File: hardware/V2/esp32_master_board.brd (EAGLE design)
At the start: 65 x 35 mm, 62 parts, among them IC1 SN74HC138PW, IC2 MAX17502EATB+T, SW1 B3U-1000P-2P-SMD

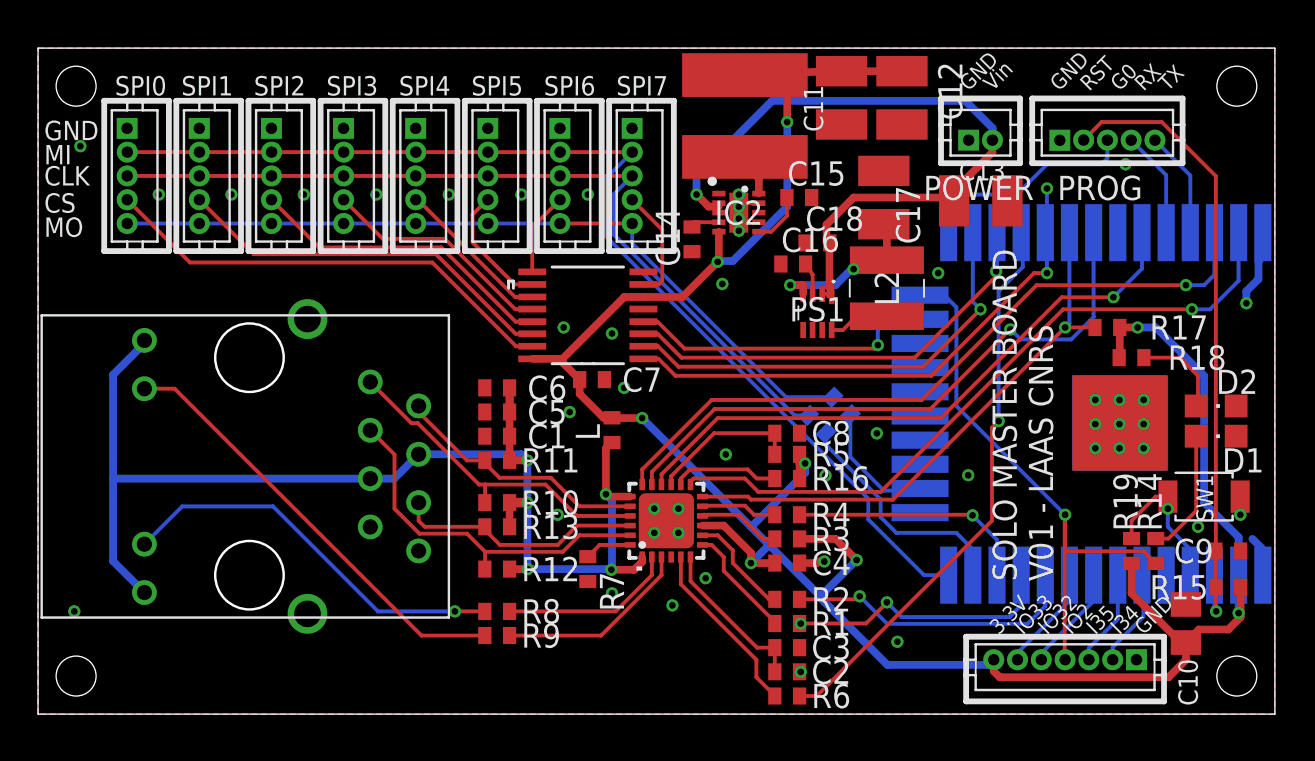
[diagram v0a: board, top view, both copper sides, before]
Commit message: [HARDWARE] Continue V2 design
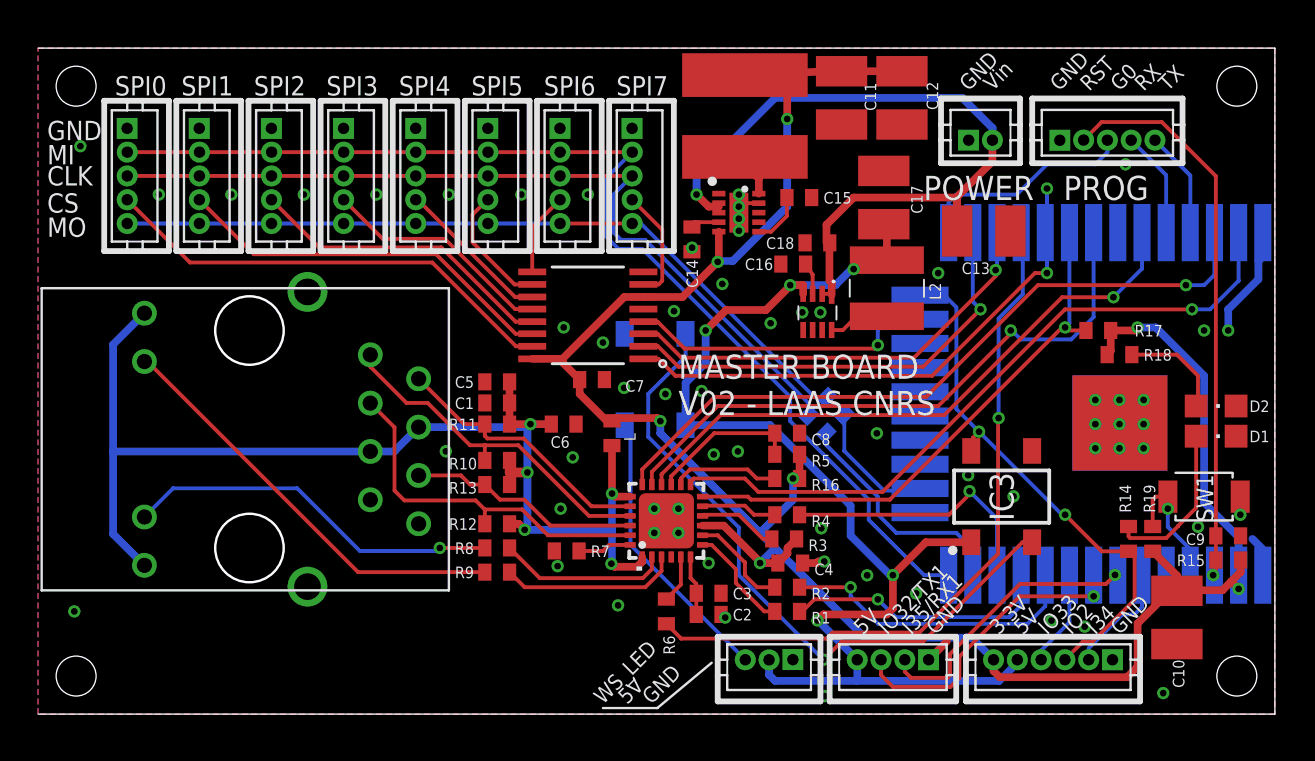
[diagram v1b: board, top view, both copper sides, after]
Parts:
- added IC3, IC4: WS2812B, WS2812B:WS2812B
- added U$5: DF13-3P-1.25DSA, con-hirose-df13:DF13-3P-1.25DSA
- added U$6: DF13-4P-1.25DSA, con-hirose-df13:DF13-4P-1.25DSA
- C10: device resistor:C0805K -> resistor:C1210
- C17: value 1u -> 22u
- U$4: value DF13-7P-1.25DSA -> DF13-6P-1.25DSA; device con-hirose-df13:DF13-7P-1.25DSA -> con-hirose-df13:DF13-6P-1.25DSA
- moved R6 7.75 mm to (33.0, 5.40), turned to 90 degrees
- moved C2 5.11 mm to (35.2, 5.24)
- moved C3 5.02 mm to (35.2, 6.35)
- moved C6 3.98 mm to (27.6, 15.2), turned to 0 degrees
- moved R8 3.33 mm to (24.1, 8.73)
- moved R9 3.33 mm to (24.1, 7.46)
- moved R12 2.38 mm to (24.1, 10.0)
- moved R10 2.22 mm to (24.1, 13.3)
- moved R13 2.22 mm to (24.1, 12.1)
- moved R11 1.90 mm to (24.1, 15.2)
- moved C1 1.75 mm to (24.1, 16.4)
- moved C13 1.60 mm to (49.7, 25.4)
- moved C5 1.59 mm to (24.1, 17.5)
- moved R14 1.56 mm to (57.3, 9.21)
- moved R7 1.46 mm to (27.8, 8.57), turned to 0 degrees
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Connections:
- removed net I35: U$1.IO35, U$4.P$3
- removed net IO32: U$1.IO32, U$4.P$5
- new net I35_RX1: U$1.IO35, U$6.P$2
- new net IO32_TX1: U$1.IO32, U$6.P$3
- new net N$19: IC3.2, IC4.4
- new net WSLED_OUT: IC4.2, U$5.P$3
- net 5V: now also IC3.1, IC4.1, U$4.P$5, U$5.P$2, U$6.P$4
- net GND: now also IC3.3, IC4.3, U$5.P$1, U$6.P$1
- net IO2: now also IC3.4, U$4.P$3; no longer U$4.P$4
- net IO33: now also U$4.P$4; no longer U$4.P$6
- net VCC: now also U$4.P$6; no longer U$4.P$7
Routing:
- net 5V: track 8.72 -> 64.1 mm, vias 2 -> 5
- net N$19: track 0.00 -> 35.3 mm, vias 0 -> 1
- net IO32_TX1: track 0.00 -> 16.0 mm, vias 0 -> 1
- net WSLED_OUT: track 0.00 -> 15.0 mm
- net I35_RX1: track 0.00 -> 14.9 mm, vias 0 -> 1
- net VCC: track 127.1 -> 118.9 mm, vias 8 -> 7
- net CLK50: track 29.8 -> 37.1 mm
- net N$5: track 9.35 -> 2.52 mm
- net IO32: track 5.58 -> 0.00 mm
- net N$14: track 8.42 -> 3.14 mm
- net I35: track 5.07 -> 0.00 mm
- net N$25: track 36.8 -> 40.6 mm
- net RST: track 33.3 -> 29.6 mm
- net GND: track 19.8 -> 22.8 mm, vias 48 -> 63
- net N$16: track 6.65 -> 8.54 mm
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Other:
- board text added: "5V"
- board text added: "I35/RX1"
- board text added: "IO32/TX1"
- board text added: "WS_LED"
- board text added: "github.com/open-dynamic-robot-initiative"
- board text removed: "I35"
- board text removed: "IO32"
- board text removed: "SOLO MASTER BOARD V01 - LAAS CNRS"
